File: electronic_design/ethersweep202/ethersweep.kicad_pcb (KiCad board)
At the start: 2 copper layers, 79 x 38 mm, 89 parts, among them J1 AVR-ISP-6, J10 HR911105A, J2 Conn_01x02_Male, J3 Conn_01x04_Female, J4 Conn_01x02_Male, J5 Conn_01x02_Male, J6 Conn_01x07_Female, J7 Conn_01x07_Male, J8 AVR-ISP-6, M1 Stepper_Motor_bipolar, SW1 SW_Push, U2 ATmega328-AU, U3 DRV8825PWPR, U4 AMS1117-3.3, U5 AS5600, U6 W5500, Y2 Crystal_25MHz, Y3 Crystal

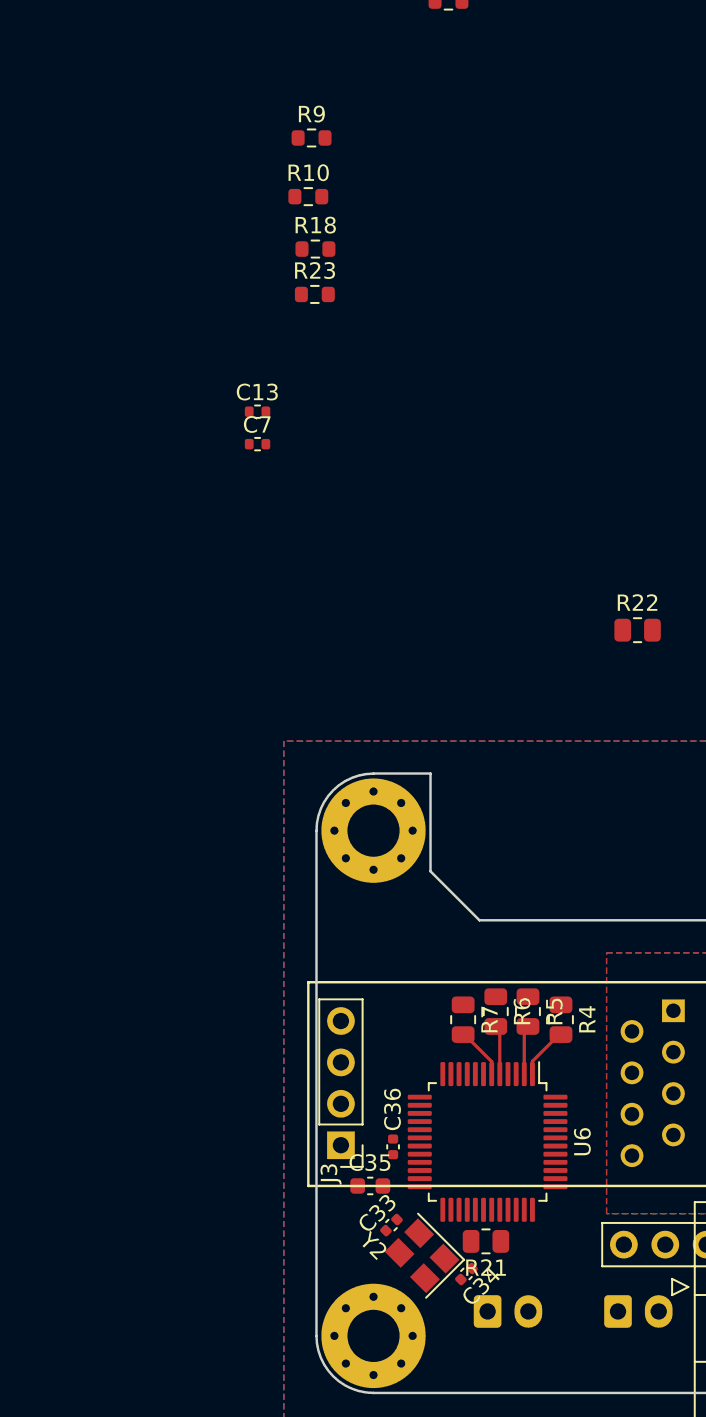
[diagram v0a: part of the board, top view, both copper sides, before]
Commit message: design and layout changes
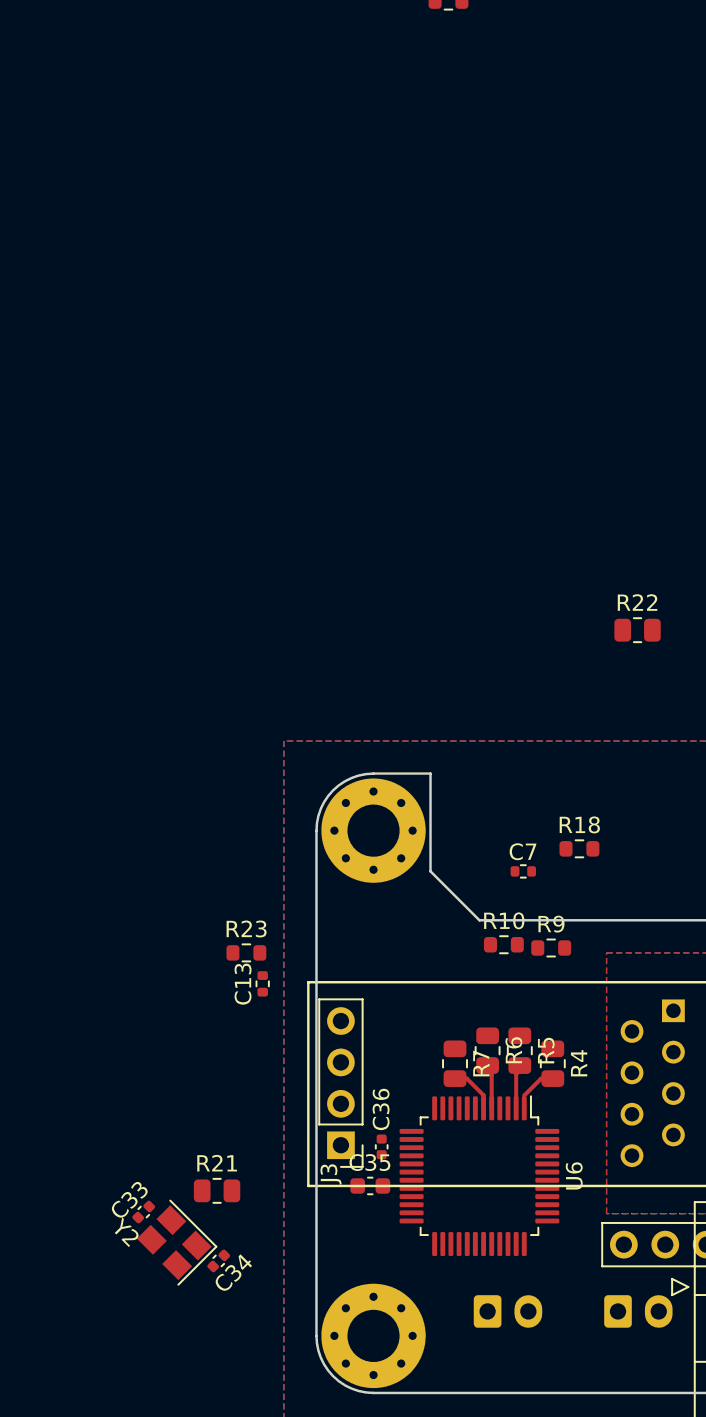
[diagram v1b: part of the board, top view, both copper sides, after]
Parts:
- moved R9 51.8 mm to (136.9, 91.7)
- moved R10 47.4 mm to (134.0, 91.5)
- moved R23 40.6 mm to (118.2, 92.0)
- moved R18 40.2 mm to (138.6, 85.6)
- moved C13 35.1 mm to (119.2, 93.9), turned to 90 degrees
- moved C7 30.9 mm to (135.2, 87.0)
- moved R21 16.8 mm to (116.4, 106.6), turned to 0 degrees
- moved Y2 15.2 mm to (113.8, 109.8)
- moved C33 15.2 mm to (111.9, 107.9)
- moved C34 15.2 mm to (116.5, 110.9)
- moved R4 2.75 mm to (137.0, 98.8)
- moved R7 2.75 mm to (131.0, 98.8)
- moved R5 2.45 mm to (135.0, 98.0)
- moved R6 2.45 mm to (133.0, 98.0)
- moved U6 2.16 mm to (132.5, 105.7)
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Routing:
- net Net-(R7-Pad2): track 3.20 -> 3.84 mm
- net Net-(R6-Pad2): track 3.03 -> 2.43 mm
- net Net-(R5-Pad2): track 3.02 -> 2.42 mm
